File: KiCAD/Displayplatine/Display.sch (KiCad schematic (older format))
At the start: 14 parts, among them P1 CONN_01X08

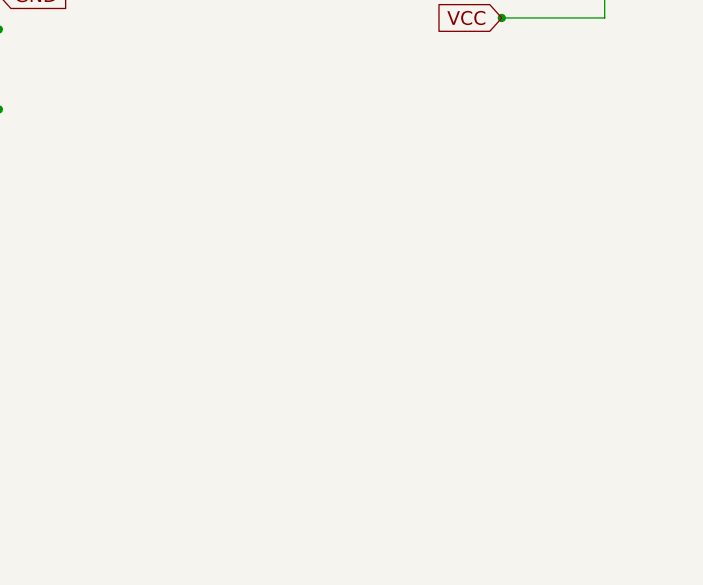
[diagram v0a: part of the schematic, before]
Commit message: Displayplatine fertig
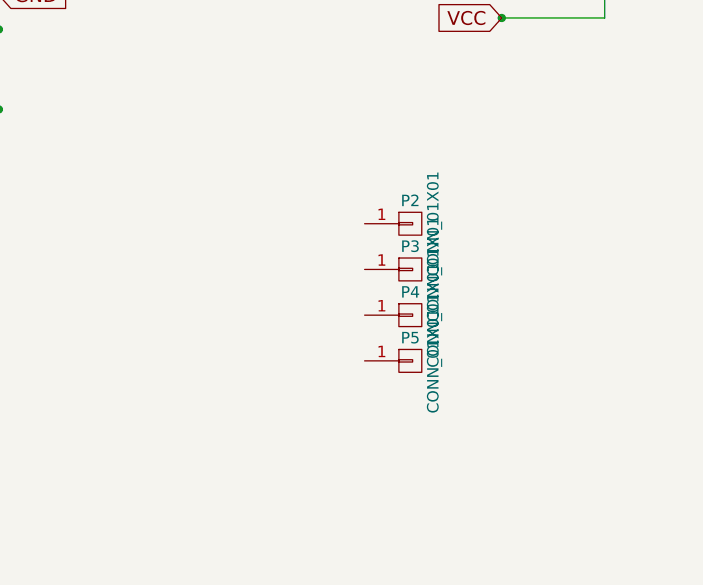
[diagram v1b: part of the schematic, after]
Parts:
- added P2, P3, P4, P5: CONN_01X01, Pin_Headers:Pin_Header_Straight_1x01, symbol CONN_01X01
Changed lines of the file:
@@
 Connection ~ 5850 3150
 Connection ~ 5850 2750
+$Comp
+L CONN_01X01 P2
+U 1 1 5630FB15
+P 7850 4450
+F 0 "P2" H 7850 4550 50  0000 C CNN
+F 1 "CONN_01X01" V 7950 4450 50  0000 C CNN
+F 2 "Pin_Headers:Pin_Header_Straight_1x01" H 7850 4450 60  0001 C CNN
+F 3 "" H 7850 4450 60  0000 C CNN
+	1    7850 4450
+	1    0    0    -1
+$EndComp
+$Comp
+L CONN_01X01 P3
+U 1 1 5630FB6B
+P 7850 4650
+F 0 "P3" H 7850 4750 50  0000 C CNN
+F 1 "CONN_01X01" V 7950 4650 50  0000 C CNN
+F 2 "Pin_Headers:Pin_Header_Straight_1x01" H 7850 4650 60  0001 C CNN
+F 3 "" H 7850 4650 60  0000 C CNN
+	1    7850 4650
+	1    0    0    -1
+$EndComp
+$Comp
+L CONN_01X01 P4
+U 1 1 5630FBB9
+P 7850 4850
+F 0 "P4" H 7850 4950 50  0000 C CNN
+F 1 "CONN_01X01" V 7950 4850 50  0000 C CNN
+F 2 "Pin_Headers:Pin_Header_Straight_1x01" H 7850 4850 60  0001 C CNN
+F 3 "" H 7850 4850 60  0000 C CNN
+	1    7850 4850
+	1    0    0    -1
+$EndComp
+$Comp
+L CONN_01X01 P5
+U 1 1 5630FC10
+P 7850 5050
+F 0 "P5" H 7850 5150 50  0000 C CNN
+F 1 "CONN_01X01" V 7950 5050 50  0000 C CNN
+F 2 "Pin_Headers:Pin_Header_Straight_1x01" H 7850 5050 60  0001 C CNN
+F 3 "" H 7850 5050 60  0000 C CNN
+	1    7850 5050
+	1    0    0    -1
+$EndComp
 $EndSCHEMATC
